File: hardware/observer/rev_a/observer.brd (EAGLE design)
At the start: 40.9 x 40.9 mm, 30 parts, among them J1 CON_HEADER_2X05-SMD+SHROUDED, J2 CON_HEADER_2X05-SMD+SHROUDED, J3 TC2030-CC2538-BL-NL, J5 PINHD-2X8/SMD, U1 LPS331AP, U2 MPU-9250, U3 SI1147, U4 SI7021, U5 ATUM, U6 AMN41121

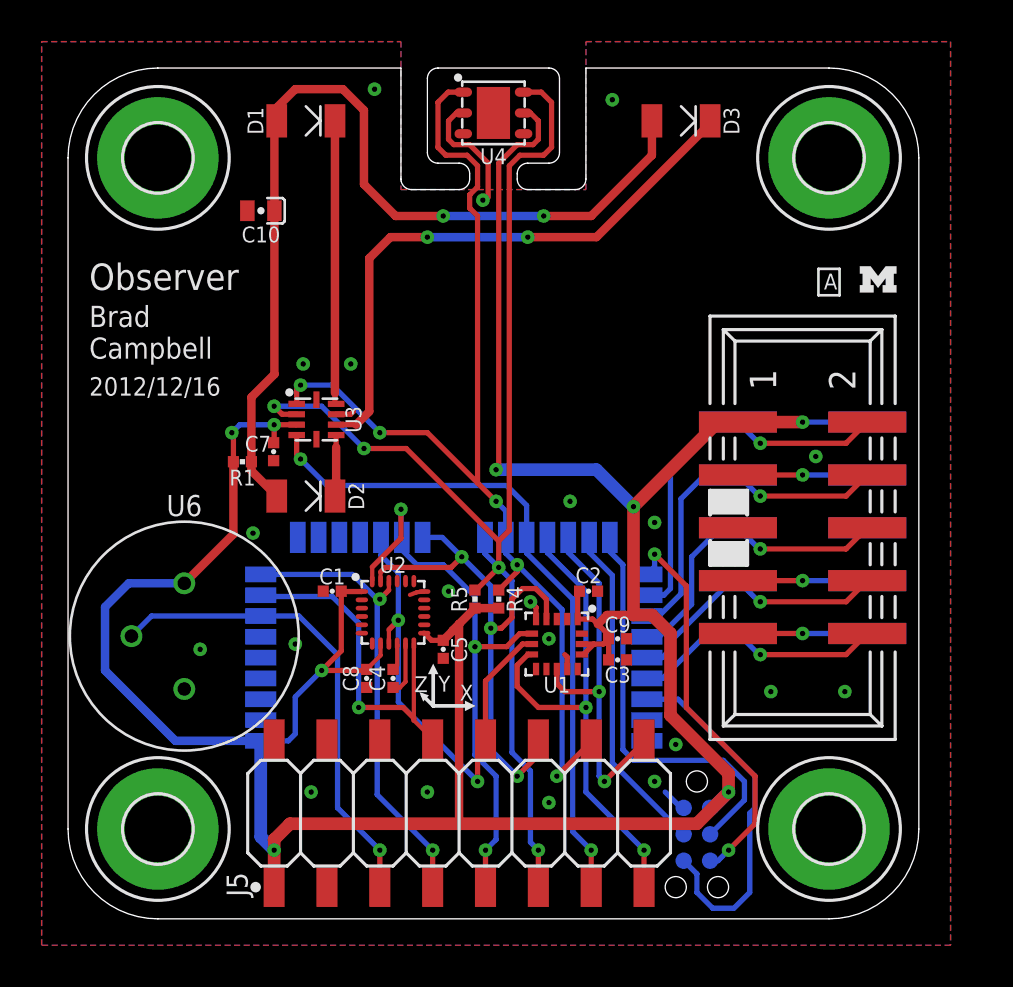
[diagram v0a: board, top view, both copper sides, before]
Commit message: shipped rev a
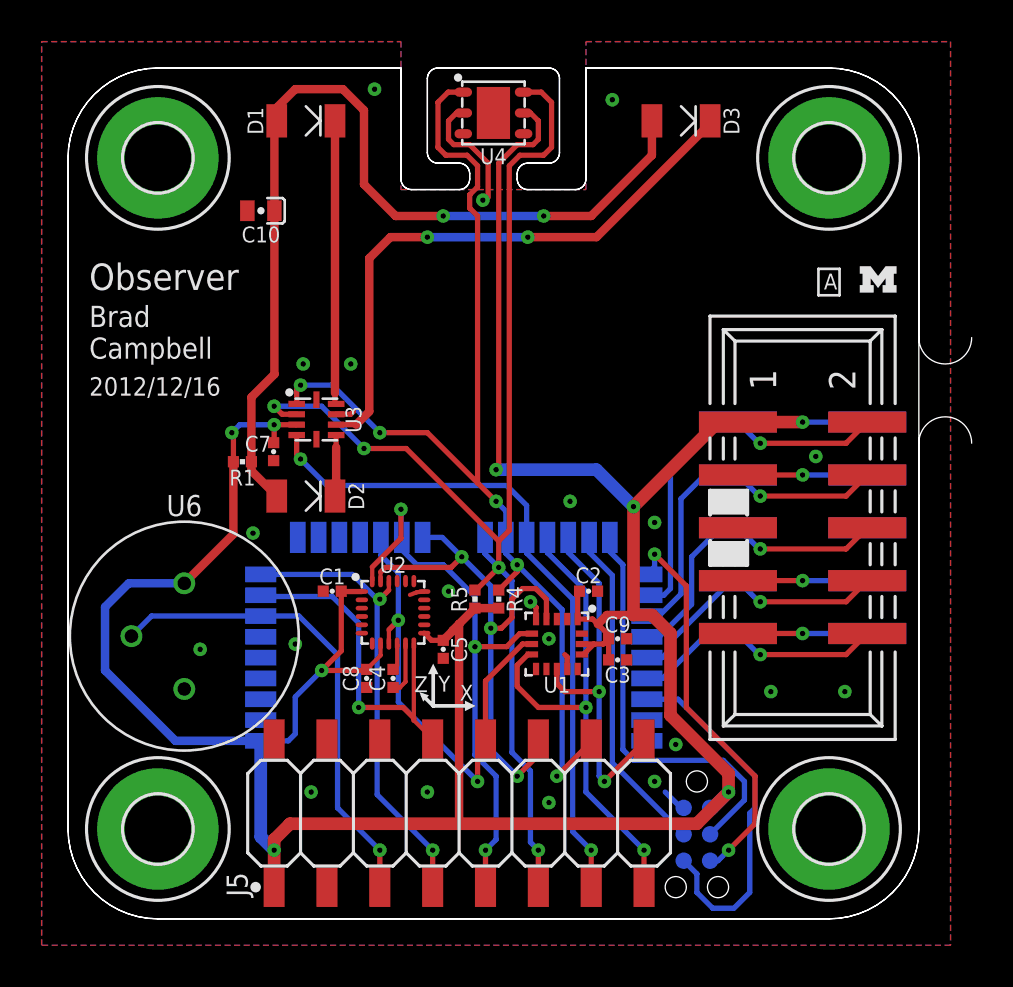
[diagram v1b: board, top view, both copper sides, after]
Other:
- board size 40.9 x 40.9 mm -> 43.4 x 40.9 mm
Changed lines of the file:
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@@
 <layer number="20" name="Dimension" color="15" fill="1" visible="yes" active="yes"/>
 <layer number="21" name="tPlace" color="7" fill="1" visible="yes" active="yes"/>
-<layer number="22" name="bPlace" color="7" fill="1" visible="yes" active="yes"/>
+<layer number="22" name="bPlace" color="7" fill="1" visible="no" active="yes"/>
 <layer number="23" name="tOrigins" color="15" fill="1" visible="yes" active="yes"/>
-<layer number="24" name="bOrigins" color="15" fill="1" visible="yes" active="yes"/>
+<layer number="24" name="bOrigins" color="15" fill="1" visible="no" active="yes"/>
 <layer number="25" name="tNames" color="7" fill="1" visible="yes" active="yes"/>
 <layer number="26" name="bNames" color="7" fill="1" visible="no" active="yes"/>
@@
 <layer number="37" name="tTest" color="7" fill="1" visible="no" active="yes"/>
 <layer number="38" name="bTest" color="7" fill="1" visible="no" active="yes"/>
-<layer number="39" name="tKeepout" color="4" fill="11" visible="yes" active="yes"/>
-<layer number="40" name="bKeepout" color="1" fill="11" visible="yes" active="yes"/>
-<layer number="41" name="tRestrict" color="4" fill="10" visible="yes" active="yes"/>
-<layer number="42" name="bRestrict" color="1" fill="10" visible="yes" active="yes"/>
-<layer number="43" name="vRestrict" color="2" fill="10" visible="yes" active="yes"/>
+<layer number="39" name="tKeepout" color="4" fill="11" visible="no" active="yes"/>
+<layer number="40" name="bKeepout" color="1" fill="11" visible="no" active="yes"/>
+<layer number="41" name="tRestrict" color="4" fill="10" visible="no" active="yes"/>
+<layer number="42" name="bRestrict" color="1" fill="10" visible="no" active="yes"/>
+<layer number="43" name="vRestrict" color="2" fill="10" visible="no" active="yes"/>
 <layer number="44" name="Drills" color="7" fill="1" visible="no" active="yes"/>
 <layer number="45" name="Holes" color="7" fill="1" visible="no" active="yes"/>
-<layer number="46" name="Milling" color="3" fill="1" visible="no" active="yes"/>
+<layer number="46" name="Milling" color="3" fill="1" visible="yes" active="yes"/>
 <layer number="47" name="Measures" color="7" fill="1" visible="no" active="yes"/>
-<layer number="48" name="Document" color="7" fill="1" visible="yes" active="yes"/>
-<layer number="49" name="Reference" color="7" fill="1" visible="yes" active="yes"/>
+<layer number="48" name="Document" color="7" fill="1" visible="no" active="yes"/>
+<layer number="49" name="Reference" color="7" fill="1" visible="no" active="yes"/>
 <layer number="50" name="dxf" color="7" fill="1" visible="no" active="no"/>
-<layer number="51" name="tDocu" color="6" fill="1" visible="yes" active="yes"/>
+<layer number="51" name="tDocu" color="6" fill="1" visible="no" active="yes"/>
 <layer number="52" name="bDocu" color="6" fill="1" visible="no" active="yes"/>
 <layer number="53" name="tGND_GNDA" color="7" fill="9" visible="no" active="no"/>
@@
 <rectangle x1="37.973" y1="19.558" x2="39.751" y2="20.574" layer="22"/>
 <rectangle x1="37.973" y1="17.018" x2="39.751" y2="18.034" layer="22"/>
+<wire x1="0" y1="36.576" x2="0" y2="4.318" width="0" layer="46"/>
+<wire x1="0" y1="4.318" x2="4.318" y2="0" width="0" layer="46" curve="90"/>
+<wire x1="4.318" y1="0" x2="36.576" y2="0" width="0" layer="46"/>
+<wire x1="36.576" y1="0" x2="40.894" y2="4.318" width="0" layer="46" curve="90"/>
+<wire x1="40.894" y1="4.318" x2="40.894" y2="22.86" width="0" layer="46"/>
+<wire x1="40.894" y1="22.86" x2="43.434" y2="22.86" width="0" layer="46" curve="-180"/>
+<wire x1="43.434" y1="27.94" x2="40.894" y2="27.94" width="0" layer="46" curve="-180"/>
+<wire x1="40.894" y1="27.94" x2="40.894" y2="36.576" width="0" layer="46"/>
+<wire x1="40.894" y1="36.576" x2="36.576" y2="40.894" width="0" layer="46" curve="90"/>
+<wire x1="4.318" y1="40.894" x2="0" y2="36.576" width="0" layer="46" curve="90"/>
+<wire x1="4.318" y1="40.894" x2="16.002" y2="40.894" width="0" layer="46"/>
+<wire x1="16.002" y1="40.894" x2="16.002" y2="35.56" width="0" layer="46"/>
+<wire x1="16.002" y1="35.56" x2="16.51" y2="35.052" width="0" layer="46" curve="90"/>
+<wire x1="16.51" y1="35.052" x2="18.796" y2="35.052" width="0" layer="46"/>
+<wire x1="18.796" y1="35.052" x2="19.304" y2="35.56" width="0" layer="46" curve="90"/>
+<wire x1="19.304" y1="35.56" x2="19.304" y2="35.814" width="0" layer="46"/>
+<wire x1="19.304" y1="35.814" x2="18.796" y2="36.322" width="0" layer="46" curve="90"/>
+<wire x1="18.796" y1="36.322" x2="17.78" y2="36.322" width="0" layer="46"/>
+<wire x1="17.78" y1="36.322" x2="17.272" y2="36.83" width="0" layer="46" curve="-90"/>
+<wire x1="17.272" y1="36.83" x2="17.272" y2="40.386" width="0" layer="46"/>
+<wire x1="17.272" y1="40.386" x2="17.78" y2="40.894" width="0" layer="46" curve="-90"/>
+<wire x1="17.78" y1="40.894" x2="23.114" y2="40.894" width="0" layer="46"/>
+<wire x1="23.114" y1="40.894" x2="23.622" y2="40.386" width="0" layer="46" curve="-90"/>
+<wire x1="23.622" y1="40.386" x2="23.622" y2="36.83" width="0" layer="46"/>
+<wire x1="23.622" y1="36.83" x2="23.114" y2="36.322" width="0" layer="46" curve="-90"/>
+<wire x1="23.114" y1="36.322" x2="22.098" y2="36.322" width="0" layer="46"/>
+<wire x1="22.098" y1="36.322" x2="21.59" y2="35.814" width="0" layer="46" curve="90"/>
+<wire x1="21.59" y1="35.814" x2="21.59" y2="35.56" width="0" layer="46"/>
+<wire x1="21.59" y1="35.56" x2="22.098" y2="35.052" width="0" layer="46" curve="90"/>
+<wire x1="22.098" y1="35.052" x2="24.384" y2="35.052" width="0" layer="46"/>
+<wire x1="24.384" y1="35.052" x2="24.892" y2="35.56" width="0" layer="46" curve="90"/>
+<wire x1="24.892" y1="35.56" x2="24.892" y2="40.894" width="0" layer="46"/>
+<wire x1="24.892" y1="40.894" x2="36.576" y2="40.894" width="0" layer="46"/>
 </plain>
 <attributes>
@@
 <param name="mlMinCreamFrame" value="0mil"/>
 <param name="mlMaxCreamFrame" value="0mil"/>
-<param name="mlViaStopLimit" value="0mil"/>
+<param name="mlViaStopLimit" value="20mil"/>
 <param name="srRoundness" value="0"/>
 <param name="srMinRoundness" value="0mil"/>
